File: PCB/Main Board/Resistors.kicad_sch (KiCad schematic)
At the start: 11 parts, among them K501 AGQ200A12, K502 AGQ200A12, K503 AGQ200A12, K504 AGQ200A12, K505 AGQ200A12

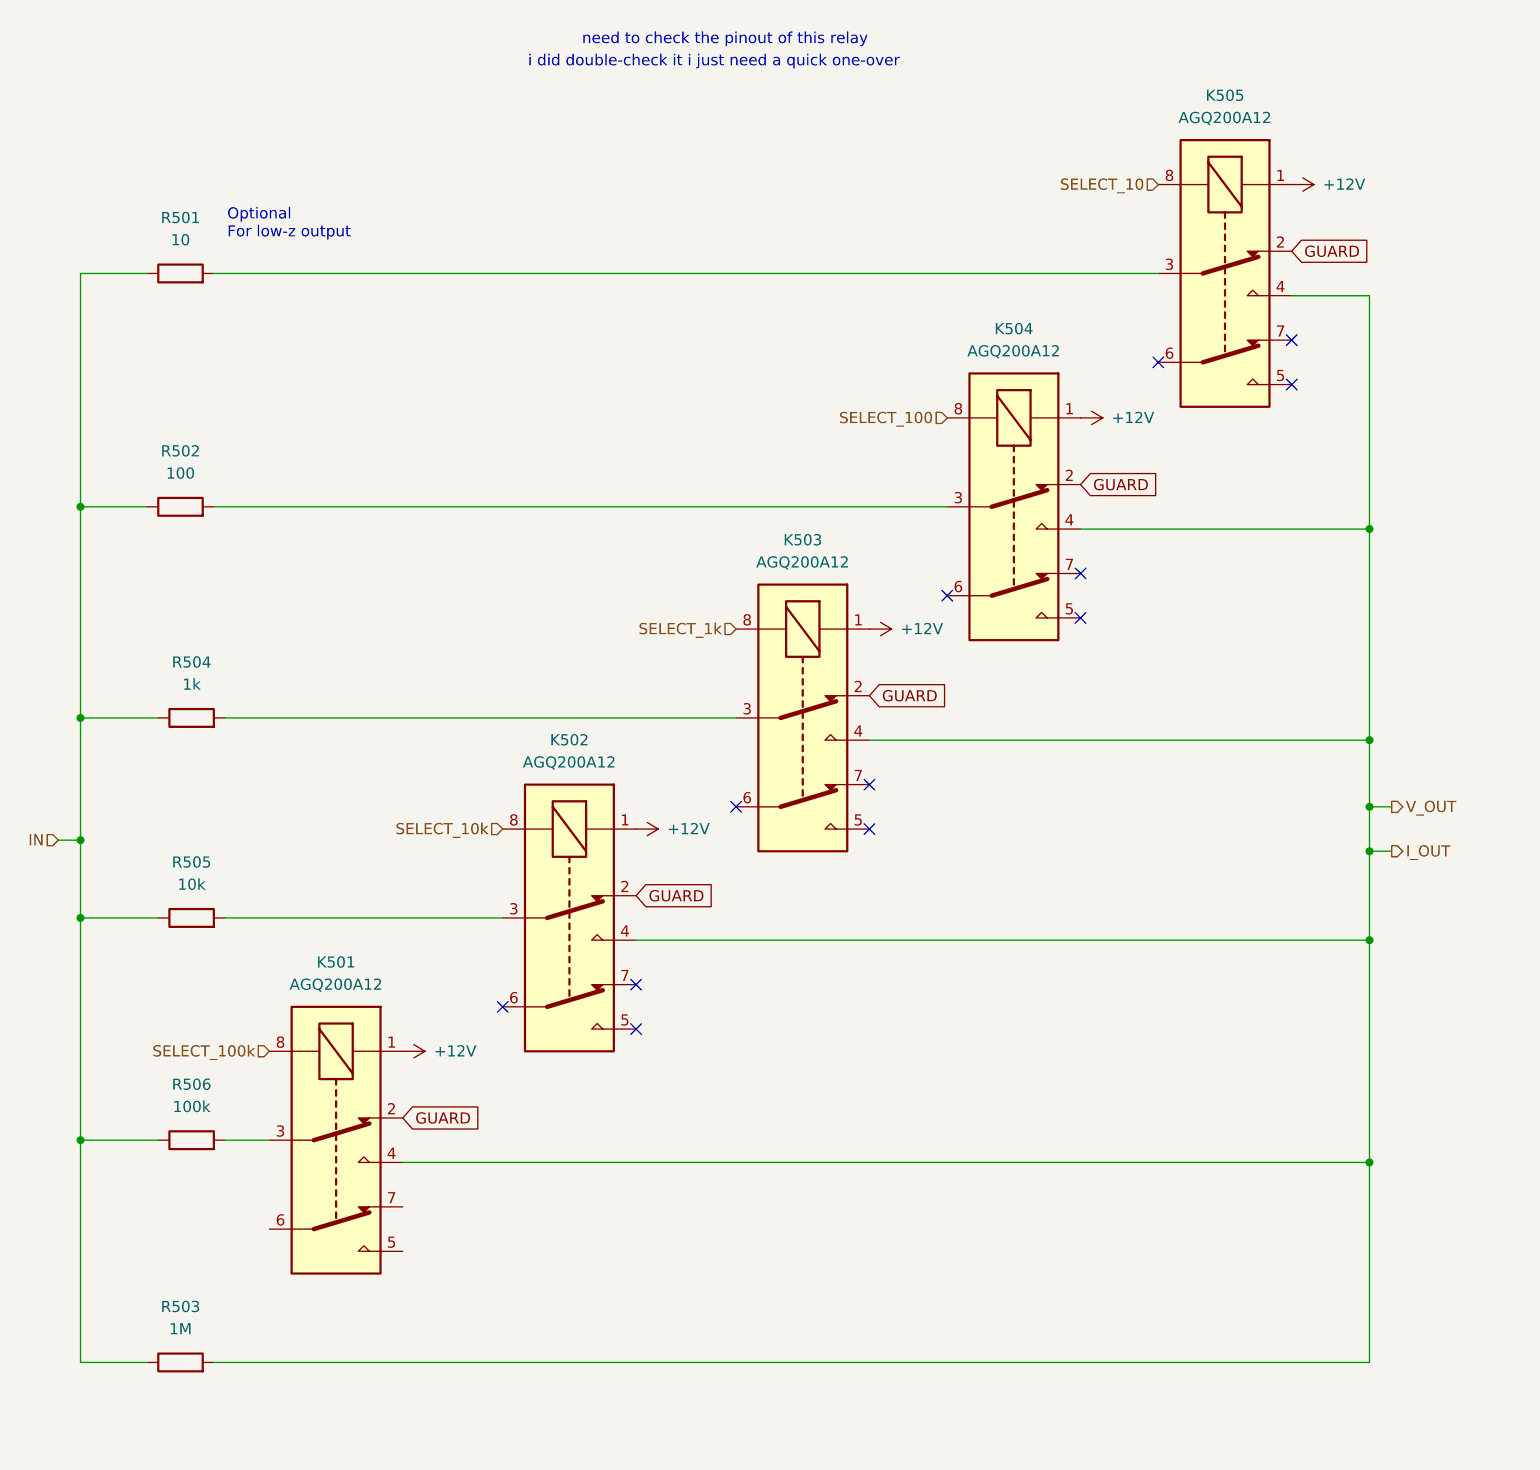
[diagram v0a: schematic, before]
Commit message: sorry i fell asleep b4 layout
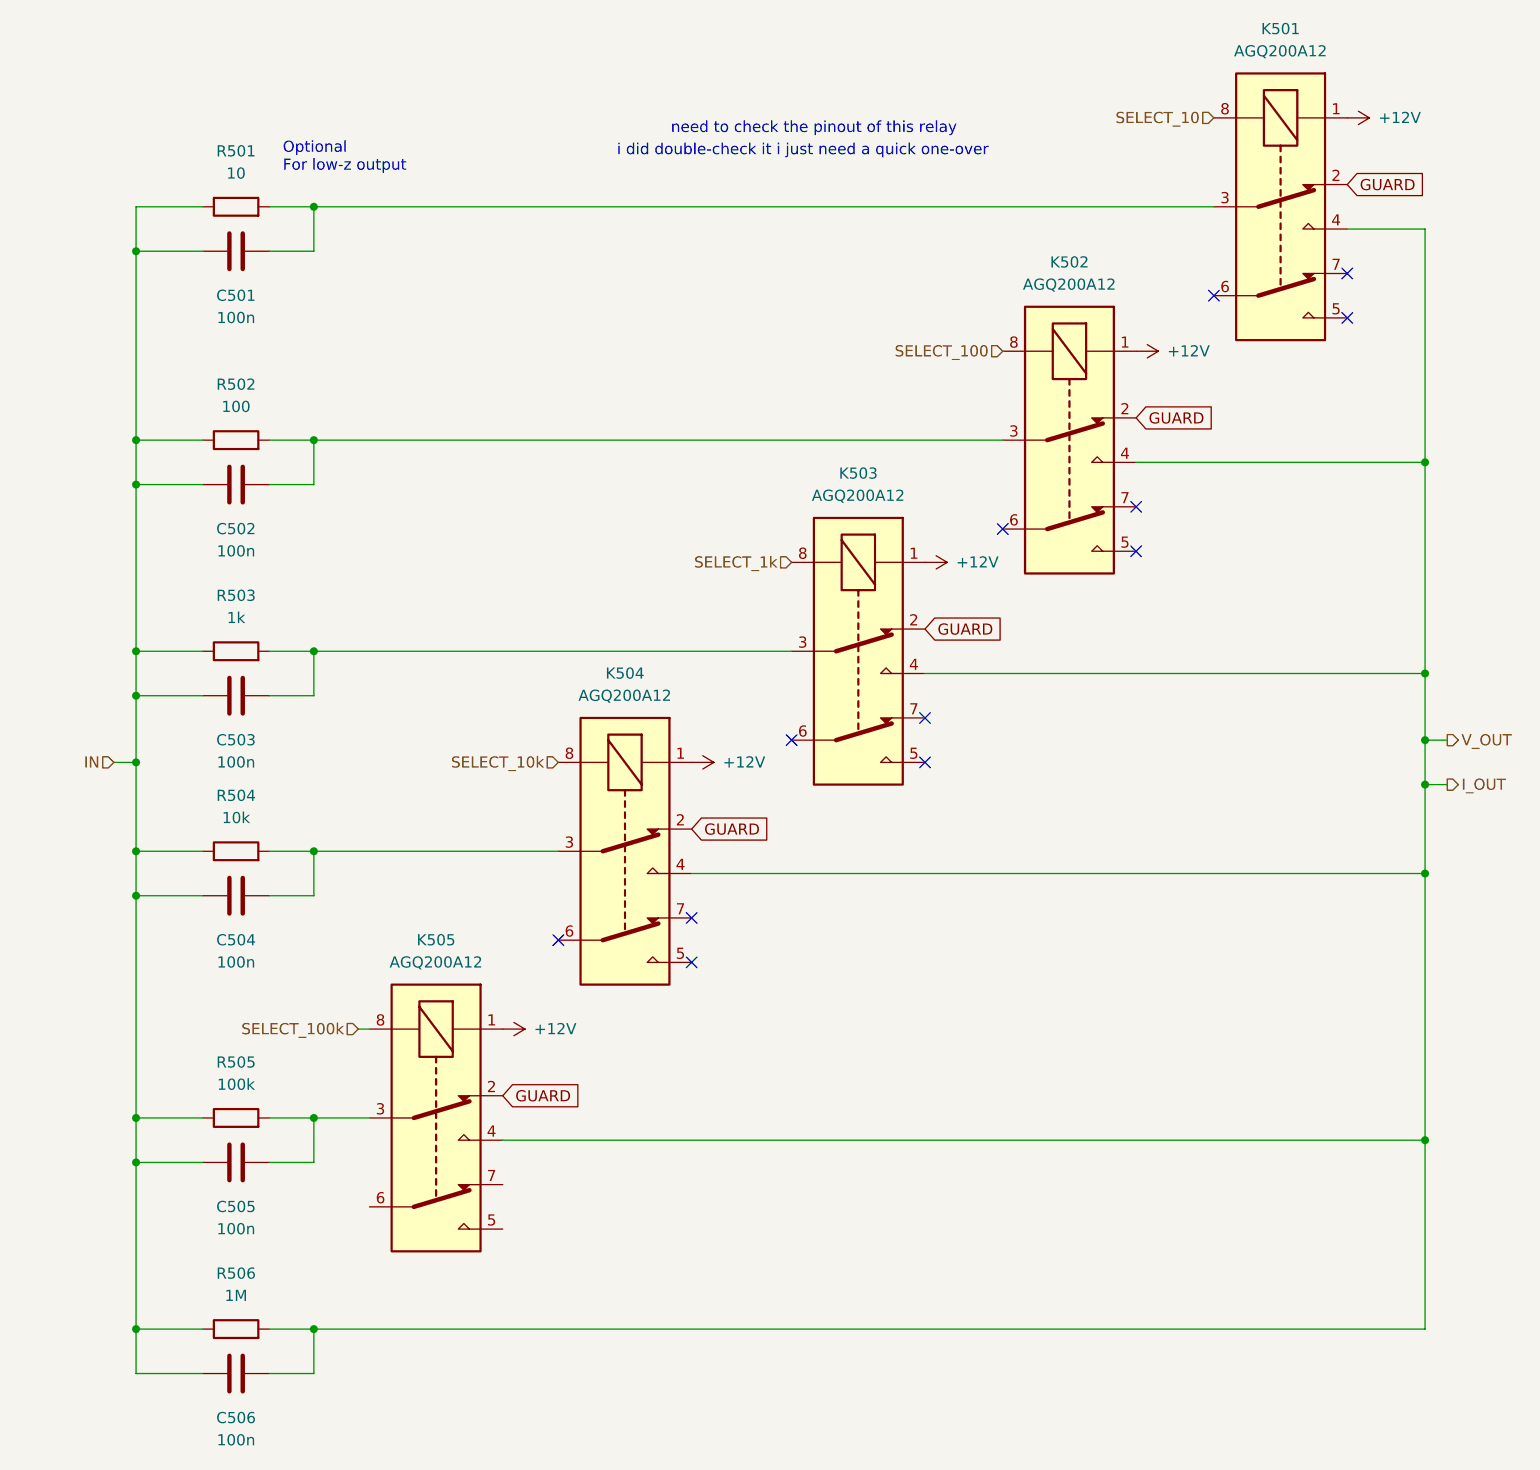
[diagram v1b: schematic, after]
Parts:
- added C501, C502, C503, C504, C505, C506: 100n, Capacitor_SMD:C_0805_2012Metric, symbol Device:C
- renumbered K505 to K501, K504 to K502, K502 to K504, K501 to K505, R504 to R503, R505 to R504, R506 to R505, R503 to R506
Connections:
- net IN: now also C501.1, C502.1, C503.1, C504.1, C505.1, C506.1
- net I_OUT: now also C506.2
- net at K503.3, R503.2: now also C503.2
- net at K501.3, R501.2: now also C501.2
- net at K502.3, R502.2: now also C502.2
- net at K505.3, R505.2: now also C505.2
- net at K504.3, R504.2: now also C504.2
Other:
- moved on the sheet: K501, K502, K503, K504, K505, R501, R502, R503, R504, R505, R506
